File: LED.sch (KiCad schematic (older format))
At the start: 17 parts

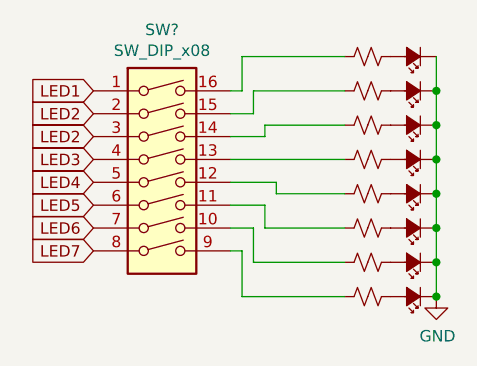
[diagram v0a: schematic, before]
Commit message: 6.bölüm
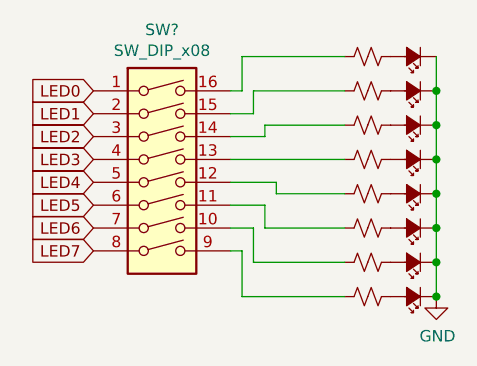
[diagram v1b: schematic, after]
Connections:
- net LED1: now also SW?.2; no longer SW?.1
- net LED2: no longer SW?.2
- new net LED0: SW?.1
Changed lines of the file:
@@
 $Descr A4 11693 8268
 encoding utf-8
-Sheet 4 6
+Sheet 4 9
 Title ""
 Date ""
@@
 Connection ~ 6450 4300
 Text GLabel 4950 3400 0    50   Input ~ 0
+LED0
+Text GLabel 4950 3500 0    50   Input ~ 0
 LED1
-Text GLabel 4950 3500 0    50   Input ~ 0
-LED2
 Text GLabel 4950 3600 0    50   Input ~ 0
 LED2
